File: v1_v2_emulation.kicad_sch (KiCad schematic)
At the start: 8 parts, among them CN5 LED, IC20 7407, IC65 D65101GD110

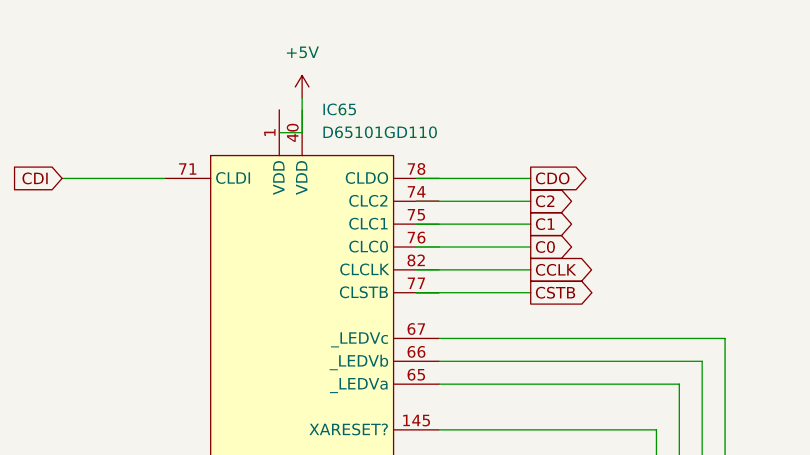
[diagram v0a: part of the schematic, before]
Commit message: fix IC65
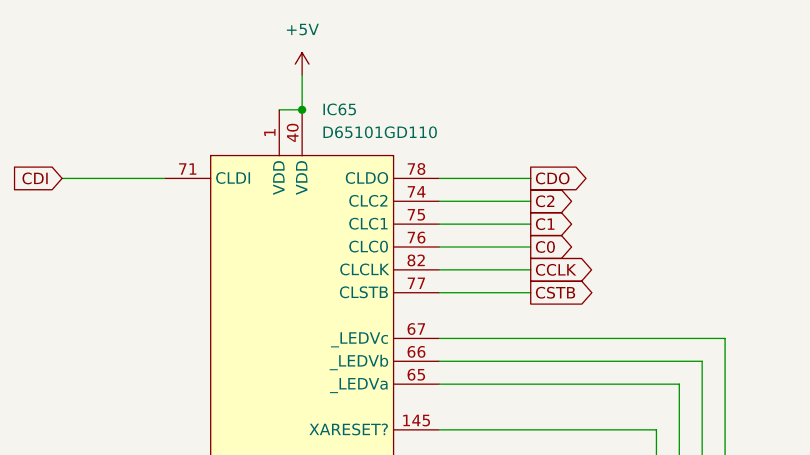
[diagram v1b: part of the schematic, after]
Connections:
- net +5V: now also IC65.1 (VDD), IC65.40 (VDD)
- net C0: now also IC65.76 (CLC0)
- net C1: now also IC65.75 (CLC1)
- net C2: now also IC65.74 (CLC2)
- net CCLK: now also IC65.82 (CLCLK)
- net CDO: now also IC65.78 (CLDO)
- net CSTB: now also IC65.77 (CLSTB)
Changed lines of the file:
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@@
   (junction (at 217.17 69.85) (diameter 0) (color 0 0 0 0)
+  )
+  (junction (at 137.16 69.85) (diameter 0) (color 0 0 0 0)
   )
   (junction (at 140.97 125.73) (diameter 0) (color 0 0 0 0)
@@
     (stroke (width 0) (type default))
   )
-  (wire (pts (xy 149.86 77.47) (xy 162.56 77.47))
+  (wire (pts (xy 152.4 77.47) (xy 162.56 77.47))
     (stroke (width 0) (type default))
   )
@@
     (stroke (width 0) (type default))
   )
-  (wire (pts (xy 137.16 68.58) (xy 137.16 72.39))
-    (stroke (width 0) (type default))
-  )
   (wire (pts (xy 217.17 69.85) (xy 234.95 69.85))
     (stroke (width 0) (type default))
@@
     (stroke (width 0) (type default))
   )
-  (wire (pts (xy 149.86 87.63) (xy 162.56 87.63))
+  (wire (pts (xy 152.4 87.63) (xy 162.56 87.63))
     (stroke (width 0) (type default))
   )
@@
     (stroke (width 0) (type default))
   )
-  (wire (pts (xy 134.62 72.39) (xy 137.16 72.39))
+  (wire (pts (xy 134.62 69.85) (xy 137.16 69.85))
     (stroke (width 0) (type default))
   )
@@
     (stroke (width 0) (type default))
   )
+  (wire (pts (xy 137.16 66.04) (xy 137.16 69.85))
+    (stroke (width 0) (type default))
+  )
   (wire (pts (xy 133.35 125.73) (xy 135.89 125.73))
     (stroke (width 0) (type default))
@@
     (stroke (width 0) (type default))
   )
-  (wire (pts (xy 149.86 82.55) (xy 162.56 82.55))
+  (wire (pts (xy 152.4 82.55) (xy 162.56 82.55))
     (stroke (width 0) (type default))
   )
@@
     (stroke (width 0) (type default))
   )
-  (wire (pts (xy 149.86 85.09) (xy 162.56 85.09))
-    (stroke (width 0) (type default))
-  )
-  (wire (pts (xy 149.86 90.17) (xy 162.56 90.17))
+  (wire (pts (xy 152.4 85.09) (xy 162.56 85.09))
+    (stroke (width 0) (type default))
+  )
+  (wire (pts (xy 152.4 90.17) (xy 162.56 90.17))
     (stroke (width 0) (type default))
   )
@@
     (stroke (width 0) (type default))
   )
-  (wire (pts (xy 149.86 80.01) (xy 162.56 80.01))
+  (wire (pts (xy 152.4 80.01) (xy 162.56 80.01))
     (stroke (width 0) (type default))
   )
@@
     (pin "2")
     (instances
-      (project "PWD665"
+      (project "88va2-circuit"
         (path "/8cd193ae-a369-4130-9ba4-f2075fa60e2b/4936267e-2afc-4e41-be53-b97a571a33d1"
           (reference "IC20") (unit 5)
@@
     (pin "2")
     (instances
-      (project "PWD665"
+      (project "88va2-circuit"
         (path "/8cd193ae-a369-4130-9ba4-f2075fa60e2b/4936267e-2afc-4e41-be53-b97a571a33d1"
           (reference "IC20") (unit 4)
@@
     (pin "67")
     (instances
-      (project "PWD665"
+      (project "88va2-circuit"
         (path "/8cd193ae-a369-4130-9ba4-f2075fa60e2b/4936267e-2afc-4e41-be53-b97a571a33d1"
           (reference "IC65") (unit 1)
@@
     )
   )
-  (symbol (lib_id "power:+5V") (at 137.16 68.58 0) (unit 1)
-    (in_bom yes) (on_board yes) (dnp no) (fields_autoplaced)
-    (property "Reference" "#PWR015" (at 137.16 72.39 0)
-      (effects (font (size 1.27 1.27)) hide)
-    )
-    (property "Value" "+5V" (at 137.16 63.5 0)
-      (effects (font (size 1.27 1.27)))
-    )
-    (property "Footprint" "" (at 137.16 68.58 0)
-      (effects (font (size 1.27 1.27)) hide)
-    )
-    (property "Datasheet" "" (at 137.16 68.58 0)
-      (effects (font (size 1.27 1.27)) hide)
-    )
-    (pin "1")
-    (instances
-      (project "PWD665"
+  (symbol (lib_id "power:+5V") (at 137.16 66.04 0) (unit 1)
+    (in_bom yes) (on_board yes) (dnp no) (fields_autoplaced)
+    (property "Reference" "#PWR015" (at 137.16 69.85 0)
+      (effects (font (size 1.27 1.27)) hide)
+    )
+    (property "Value" "+5V" (at 137.16 60.96 0)
+      (effects (font (size 1.27 1.27)))
+    )
+    (property "Footprint" "" (at 137.16 66.04 0)
+      (effects (font (size 1.27 1.27)) hide)
+    )
+    (property "Datasheet" "" (at 137.16 66.04 0)
+      (effects (font (size 1.27 1.27)) hide)
+    )
+    (pin "1")
+    (instances
+      (project "88va2-circuit"
         (path "/8cd193ae-a369-4130-9ba4-f2075fa60e2b/4936267e-2afc-4e41-be53-b97a571a33d1"
           (reference "#PWR015") (unit 1)
@@
     (pin "2")
     (instances
-      (project "PWD665"
+      (project "88va2-circuit"
         (path "/8cd193ae-a369-4130-9ba4-f2075fa60e2b/4936267e-2afc-4e41-be53-b97a571a33d1"
           (reference "IC20") (unit 3)
@@
     (pin "1")
     (instances
-      (project "PWD665"
+      (project "88va2-circuit"
         (path "/8cd193ae-a369-4130-9ba4-f2075fa60e2b/4936267e-2afc-4e41-be53-b97a571a33d1"
           (reference "C66") (unit 1)
@@
     (pin "2")
     (instances
-      (project "PWD665"
+      (project "88va2-circuit"
         (path "/8cd193ae-a369-4130-9ba4-f2075fa60e2b/4936267e-2afc-4e41-be53-b97a571a33d1"
           (reference "IC20") (unit 2)
@@
     (pin "2")
     (instances
-      (project "PWD665"
+      (project "88va2-circuit"
         (path "/8cd193ae-a369-4130-9ba4-f2075fa60e2b/4936267e-2afc-4e41-be53-b97a571a33d1"
           (reference "IC20") (unit 7)
@@
     (pin "3")
     (instances
-      (project "PWD665"
+      (project "88va2-circuit"
         (path "/8cd193ae-a369-4130-9ba4-f2075fa60e2b/4936267e-2afc-4e41-be53-b97a571a33d1"
           (reference "LC7") (unit 1)
@@
     (pin "1")
     (instances
-      (project "PWD665"
+      (project "88va2-circuit"
         (path "/8cd193ae-a369-4130-9ba4-f2075fa60e2b/4936267e-2afc-4e41-be53-b97a571a33d1"
           (reference "#PWR021") (unit 1)
@@
     (pin "2")
     (instances
-      (project "PWD665"
+      (project "88va2-circuit"
         (path "/8cd193ae-a369-4130-9ba4-f2075fa60e2b/4936267e-2afc-4e41-be53-b97a571a33d1"
           (reference "IC20") (unit 6)
@@
     (pin "1")
     (instances
-      (project "PWD665"
+      (project "88va2-circuit"
         (path "/8cd193ae-a369-4130-9ba4-f2075fa60e2b/4936267e-2afc-4e41-be53-b97a571a33d1"
           (reference "#PWR020") (unit 1)
@@
     (pin "3")
     (instances
-      (project "PWD665"
+      (project "88va2-circuit"
         (path "/8cd193ae-a369-4130-9ba4-f2075fa60e2b/4936267e-2afc-4e41-be53-b97a571a33d1"
           (reference "LC6") (unit 1)
@@
     (pin "1")
     (instances
-      (project "PWD665"
+      (project "88va2-circuit"
         (path "/8cd193ae-a369-4130-9ba4-f2075fa60e2b/4936267e-2afc-4e41-be53-b97a571a33d1"
           (reference "#PWR016") (unit 1)
@@
     (pin "2")
     (instances
-      (project "PWD665"
+      (project "88va2-circuit"
         (path "/8cd193ae-a369-4130-9ba4-f2075fa60e2b/4936267e-2afc-4e41-be53-b97a571a33d1"
           (reference "IC20") (unit 1)
@@
     (pin "1")
     (instances
-      (project "PWD665"
+      (project "88va2-circuit"
         (path "/8cd193ae-a369-4130-9ba4-f2075fa60e2b/4936267e-2afc-4e41-be53-b97a571a33d1"
           (reference "#PWR022") (unit 1)
@@
     (pin "1")
     (instances
-      (project "PWD665"
+      (project "88va2-circuit"
         (path "/8cd193ae-a369-4130-9ba4-f2075fa60e2b/4936267e-2afc-4e41-be53-b97a571a33d1"
           (reference "#PWR024") (unit 1)
@@
     (pin "1")
     (instances
-      (project "PWD665"
+      (project "88va2-circuit"
         (path "/8cd193ae-a369-4130-9ba4-f2075fa60e2b/4936267e-2afc-4e41-be53-b97a571a33d1"
           (reference "#PWR019") (unit 1)
@@
     (pin "1")
     (instances
-      (project "PWD665"
+      (project "88va2-circuit"
         (path "/8cd193ae-a369-4130-9ba4-f2075fa60e2b/4936267e-2afc-4e41-be53-b97a571a33d1"
           (reference "#PWR014") (unit 1)
@@
     (pin "3")
     (instances
-      (project "PWD665"
+      (project "88va2-circuit"
         (path "/8cd193ae-a369-4130-9ba4-f2075fa60e2b/4936267e-2afc-4e41-be53-b97a571a33d1"
           (reference "LC8") (unit 1)
@@
     (pin "3")
     (instances
-      (project "PWD665"
+      (project "88va2-circuit"
         (path "/8cd193ae-a369-4130-9ba4-f2075fa60e2b/4936267e-2afc-4e41-be53-b97a571a33d1"
           (reference "LC23") (unit 1)
@@
     (pin "2")
     (instances
-      (project "PWD665"
+      (project "88va2-circuit"
         (path "/8cd193ae-a369-4130-9ba4-f2075fa60e2b/4936267e-2afc-4e41-be53-b97a571a33d1"
           (reference "CN5") (unit 1)
@@
     (pin "1")
     (instances
-      (project "PWD665"
+      (project "88va2-circuit"
         (path "/8cd193ae-a369-4130-9ba4-f2075fa60e2b/4936267e-2afc-4e41-be53-b97a571a33d1"
           (reference "#PWR017") (unit 1)
@@
     (pin "1")
     (instances
-      (project "PWD665"
+      (project "88va2-circuit"
         (path "/8cd193ae-a369-4130-9ba4-f2075fa60e2b/4936267e-2afc-4e41-be53-b97a571a33d1"
           (reference "#PWR018") (unit 1)
